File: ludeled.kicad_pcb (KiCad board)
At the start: 2 copper layers, 379 parts, among them U1 ESP32-WROOM-32E

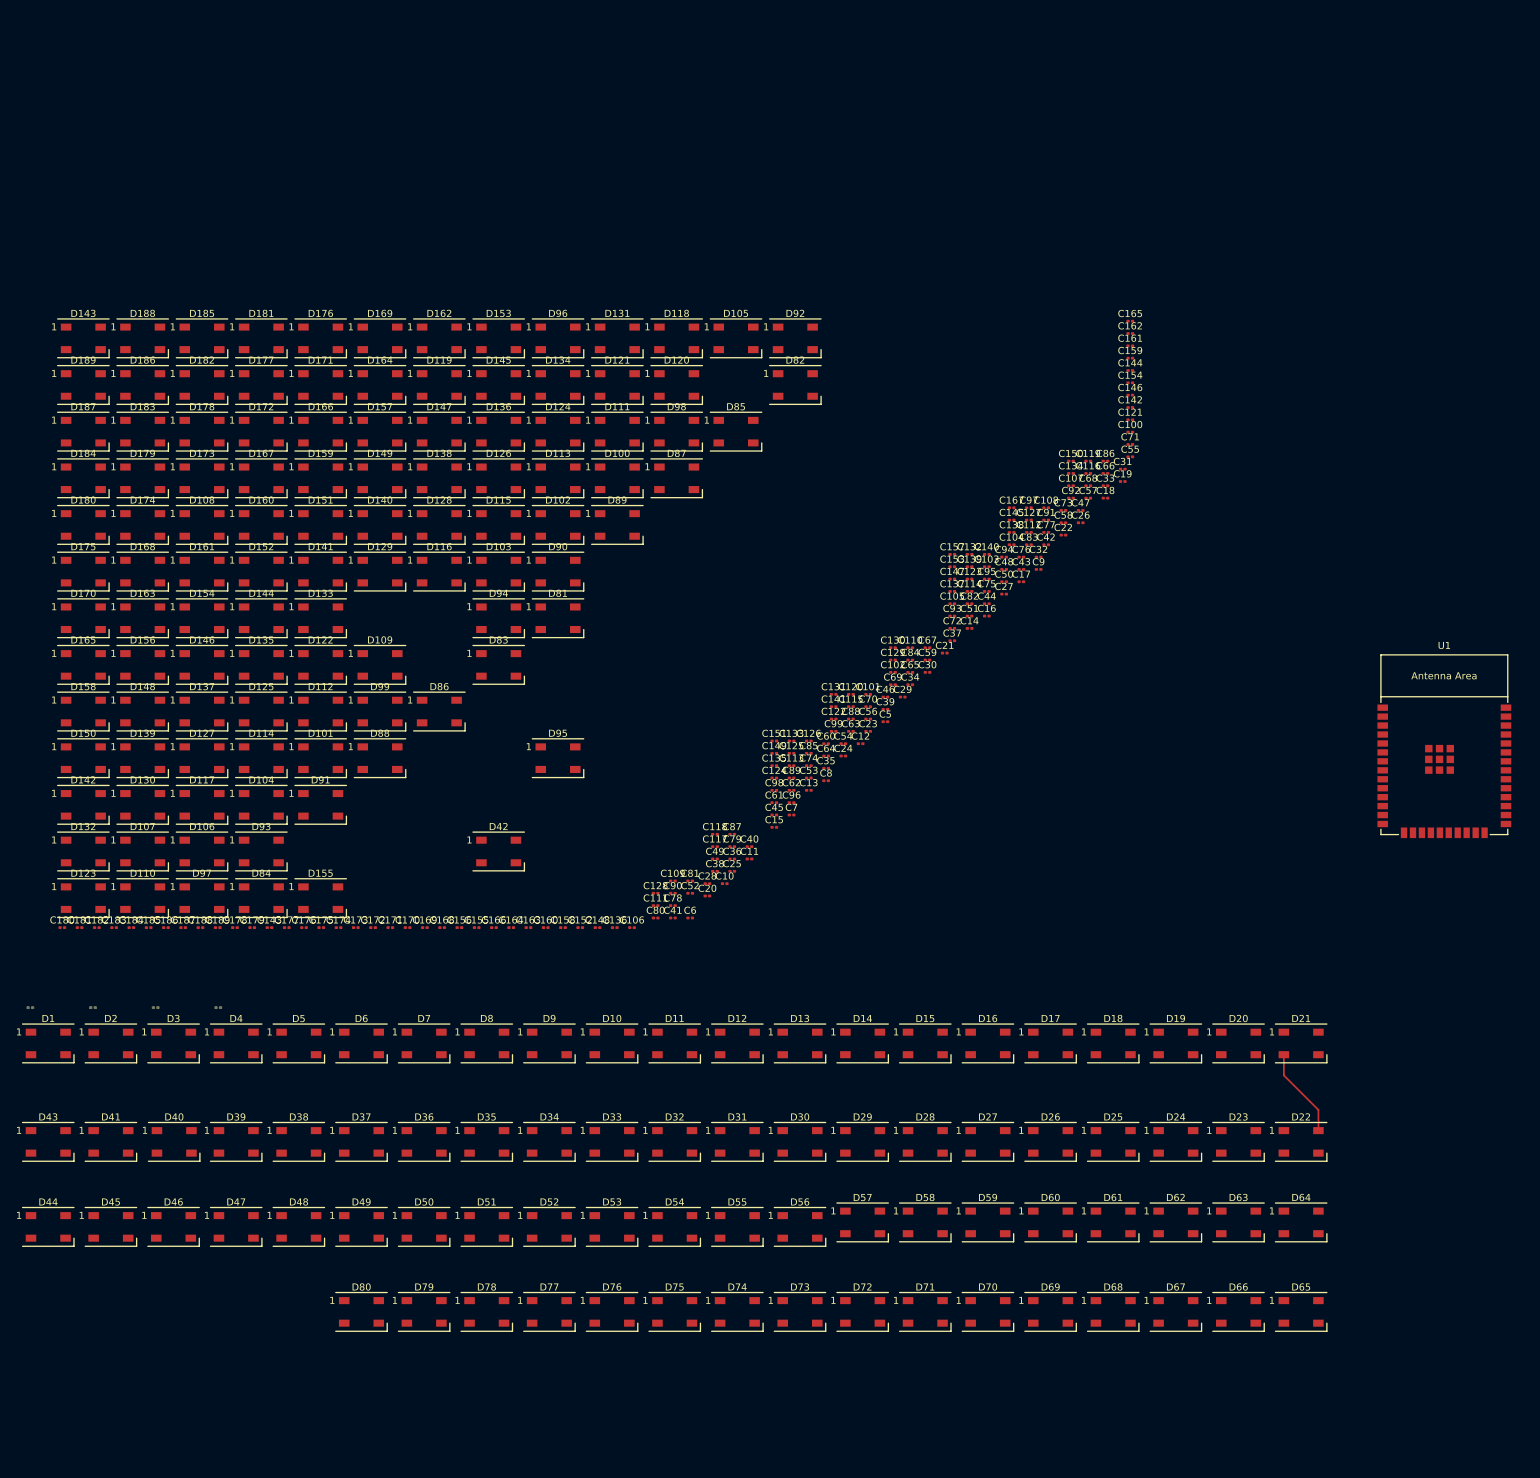
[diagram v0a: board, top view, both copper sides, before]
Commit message: More layout
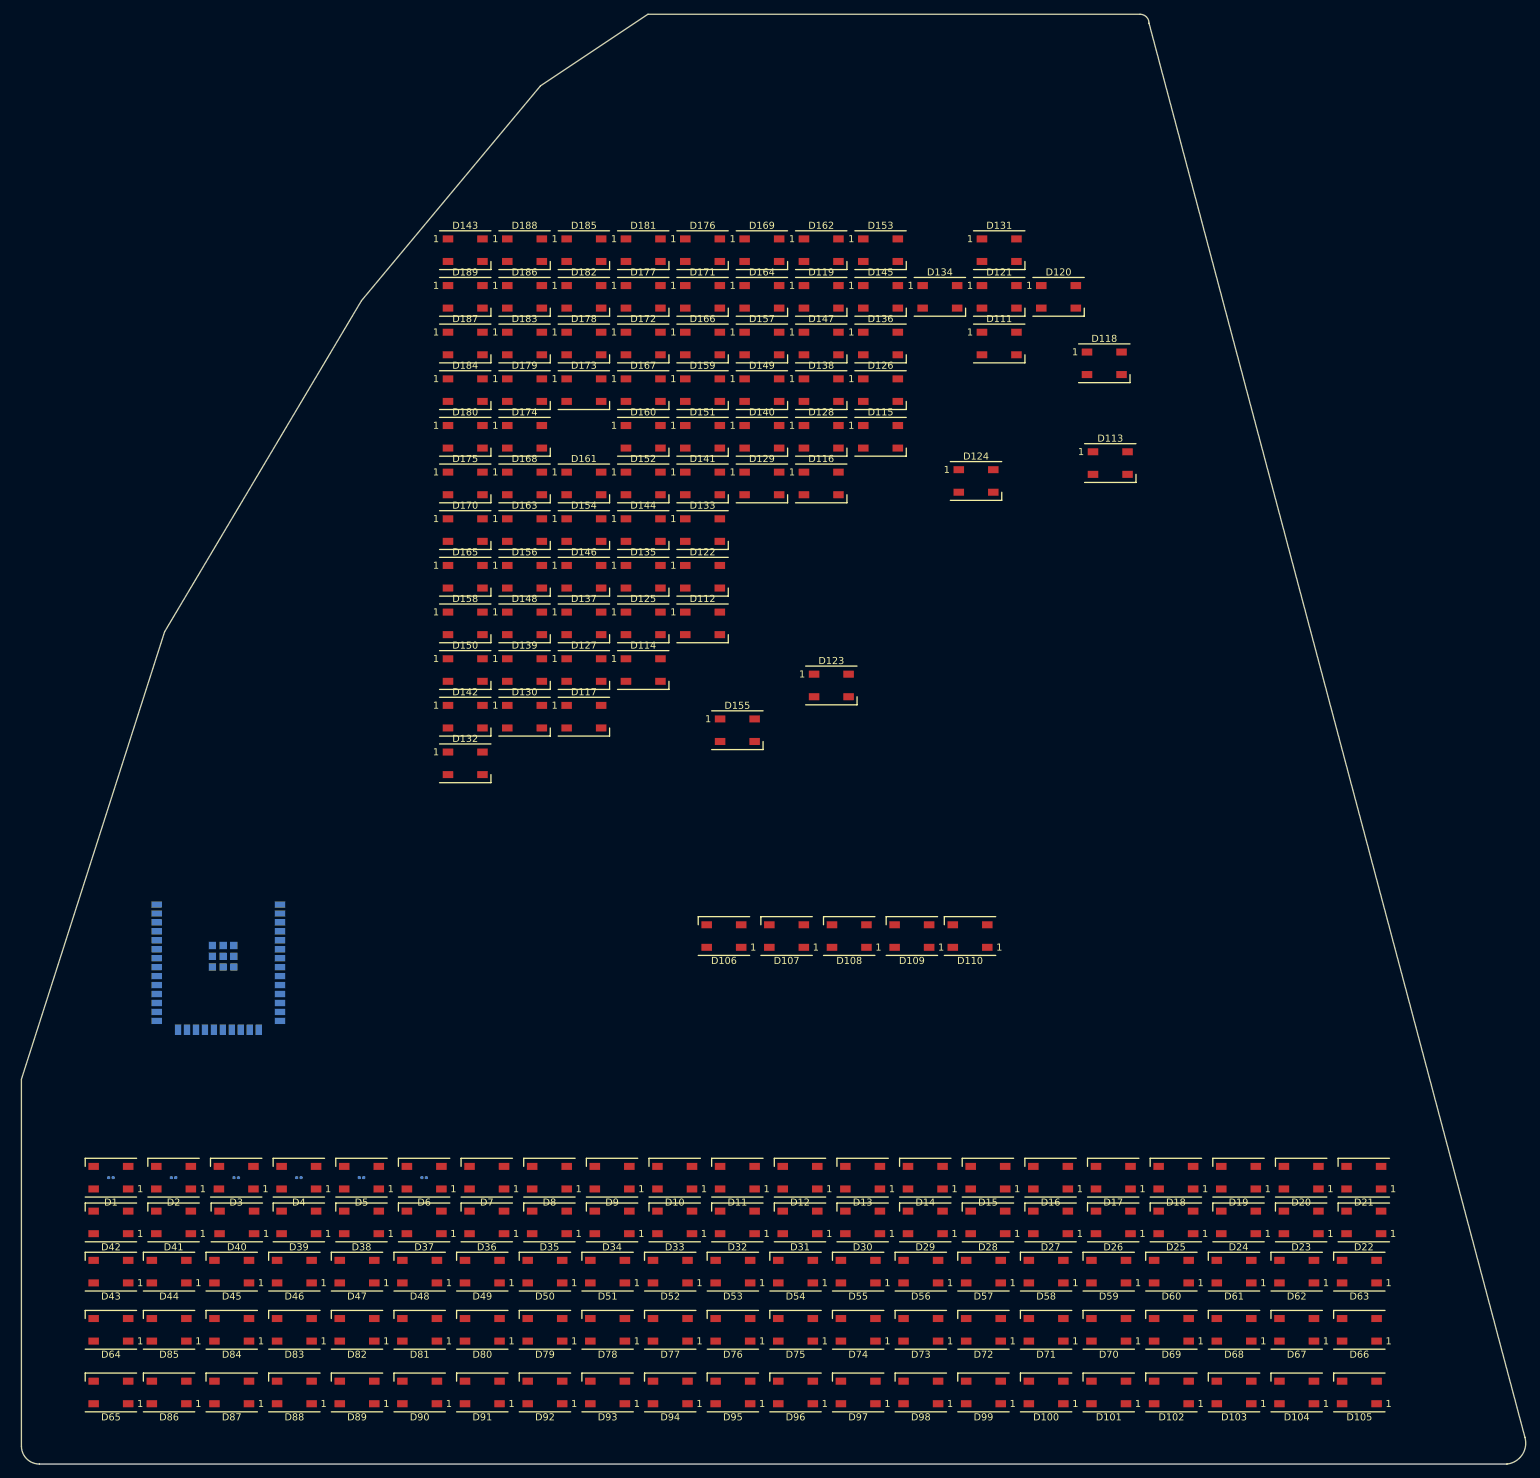
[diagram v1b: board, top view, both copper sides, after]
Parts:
- removed C10, C100, C101, C102, C103, C104, C105, C106, C107, C108, C109, C11, C110, C111, C112, C113, C114, C115, C116, C117, C118, C119, C12, C120, C121, C122, C123, C124, C125, C126, C127, C128, C129, C13, C130, C131, C132, C133, C134, C135, C136, C137, C138, C139, C14, C140, C141, C142, C143, C144, C145, C146, C147, C148, C149, C15, C150, C151, C152, C153, C154, C155, C156, C157, C158, C159, C16, C160, C161, C162, C163, C164, C165, C166, C167, C168, C169, C17, C170, C171, C172, C173, C174, C175, C176, C177, C178, C179, C18, C180, C181, C182, C183, C184, C185, C186, C187, C188, C189, C19, C20, C21, C22, C23, C24, C25, C26, C27, C28, C29, C30, C31, C32, C33, C34, C35, C36, C37, C38, C39, C40, C41, C42, C43, C44, C45, C46, C47, C48, C49, C50, C51, C52, C53, C54, C55, C56, C57, C58, C59, C60, C61, C62, C63, C64, C65, C66, C67, C68, C69, C7, C70, C71, C72, C73, C74, C75, C76, C77, C78, C79, C8, C80, C81, C82, C83, C84, C85, C86, C87, C88, C89, C9, C90, C91, C92, C93, C94, C95, C96, C97, C98, C99: 100nF, Capacitor_SMD:C_0201_0603Metric
- C5, C6, U1: moved to B.Cu
- moved U1 176.2 mm to (64.8, 74.9), turned to 180 degrees
- moved D105 173.8 mm to (226.7, 137.2), turned to 180 degrees
- moved D64 169.6 mm to (49.5, 128.3), turned to 180 degrees
- moved D65 169.3 mm to (49.5, 137.2), turned to 180 degrees
- moved D104 168.9 mm to (217.8, 137.2), turned to 180 degrees
- moved D103 156.4 mm to (208.9, 137.2), turned to 180 degrees
- moved D92 153.8 mm to (111.1, 137.2), turned to 180 degrees
- moved D96 153.3 mm to (146.7, 137.2), turned to 180 degrees
- moved D102 150.8 mm to (200.0, 137.2), turned to 180 degrees
- moved D85 150.7 mm to (57.8, 128.3), turned to 180 degrees
- moved D82 147.8 mm to (84.5, 128.3), turned to 180 degrees
- moved D87 144.3 mm to (66.7, 137.2), turned to 180 degrees
- moved D101 143.6 mm to (191.1, 137.2), turned to 180 degrees
- moved D100 143.3 mm to (182.2, 137.2), turned to 180 degrees
- moved D98 140.7 mm to (164.5, 137.2), turned to 180 degrees
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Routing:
- net Net-(D21-Pad2): track 12.8 -> 0.00 mm
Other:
- board outline added: 213.5 x 205.7 mm

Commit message: layout done
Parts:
- added C7: 100nF, Capacitor_SMD:C_0201_0603Metric, F.Cu at (134.1, 16.8)
- added C8: 100nF, Capacitor_SMD:C_0201_0603Metric, F.Cu at (142.3, 16.8)
- added C9: 100nF, Capacitor_SMD:C_0201_0603Metric, F.Cu at (150.7, 16.8)
- added D190: WS2812B, LED_SMD:LED_WS2812B_PLCC4_5.0x5.0mm_P3.2mm, F.Cu at (98.5, 113.0)
- added D191: WS2812B, LED_SMD:LED_WS2812B_PLCC4_5.0x5.0mm_P3.2mm, F.Cu at (106.8, 113.0)
- added D192: WS2812B, LED_SMD:LED_WS2812B_PLCC4_5.0x5.0mm_P3.2mm, F.Cu at (115.0, 113.0)
- added D193: WS2812B, LED_SMD:LED_WS2812B_PLCC4_5.0x5.0mm_P3.2mm, F.Cu at (123.2, 113.0)
- added D194: WS2812B, LED_SMD:LED_WS2812B_PLCC4_5.0x5.0mm_P3.2mm, F.Cu at (131.5, 113.0)
- added D195: WS2812B, LED_SMD:LED_WS2812B_PLCC4_5.0x5.0mm_P3.2mm, F.Cu at (139.8, 113.0)
- added D196: WS2812B, LED_SMD:LED_WS2812B_PLCC4_5.0x5.0mm_P3.2mm, F.Cu at (148.0, 113.0)
- added D197: WS2812B, LED_SMD:LED_WS2812B_PLCC4_5.0x5.0mm_P3.2mm, F.Cu at (156.2, 113.0)
- added D198: WS2812B, LED_SMD:LED_WS2812B_PLCC4_5.0x5.0mm_P3.2mm, F.Cu at (164.5, 113.0)
- added D199: WS2812B, LED_SMD:LED_WS2812B_PLCC4_5.0x5.0mm_P3.2mm, F.Cu at (172.8, 113.0)
- added D200: WS2812B, LED_SMD:LED_WS2812B_PLCC4_5.0x5.0mm_P3.2mm, F.Cu at (7.50, 121.2)
- added D201: WS2812B, LED_SMD:LED_WS2812B_PLCC4_5.0x5.0mm_P3.2mm, F.Cu at (15.8, 121.2)
- added D202: WS2812B, LED_SMD:LED_WS2812B_PLCC4_5.0x5.0mm_P3.2mm, F.Cu at (24.0, 121.2)
- added D203: WS2812B, LED_SMD:LED_WS2812B_PLCC4_5.0x5.0mm_P3.2mm, F.Cu at (32.2, 121.2)
- added D204: WS2812B, LED_SMD:LED_WS2812B_PLCC4_5.0x5.0mm_P3.2mm, F.Cu at (40.5, 121.2)
- added D205: WS2812B, LED_SMD:LED_WS2812B_PLCC4_5.0x5.0mm_P3.2mm, F.Cu at (48.8, 121.2)
- added D206: WS2812B, LED_SMD:LED_WS2812B_PLCC4_5.0x5.0mm_P3.2mm, F.Cu at (57.0, 121.2)
- added D207: WS2812B, LED_SMD:LED_WS2812B_PLCC4_5.0x5.0mm_P3.2mm, F.Cu at (65.2, 121.2)
- added D208: WS2812B, LED_SMD:LED_WS2812B_PLCC4_5.0x5.0mm_P3.2mm, F.Cu at (73.5, 121.2)
- added D209: WS2812B, LED_SMD:LED_WS2812B_PLCC4_5.0x5.0mm_P3.2mm, F.Cu at (81.8, 121.2)
- added D210: WS2812B, LED_SMD:LED_WS2812B_PLCC4_5.0x5.0mm_P3.2mm, F.Cu at (90.0, 121.2)
- added D211: WS2812B, LED_SMD:LED_WS2812B_PLCC4_5.0x5.0mm_P3.2mm, F.Cu at (98.2, 121.2)
- added D212: WS2812B, LED_SMD:LED_WS2812B_PLCC4_5.0x5.0mm_P3.2mm, F.Cu at (106.5, 121.2)
- added D213: WS2812B, LED_SMD:LED_WS2812B_PLCC4_5.0x5.0mm_P3.2mm, F.Cu at (115.0, 121.2)
- added D214: WS2812B, LED_SMD:LED_WS2812B_PLCC4_5.0x5.0mm_P3.2mm, F.Cu at (123.2, 121.2)
- added D215: WS2812B, LED_SMD:LED_WS2812B_PLCC4_5.0x5.0mm_P3.2mm, F.Cu at (131.8, 121.2)
- added D216: WS2812B, LED_SMD:LED_WS2812B_PLCC4_5.0x5.0mm_P3.2mm, F.Cu at (140.0, 121.2)
- added D217: WS2812B, LED_SMD:LED_WS2812B_PLCC4_5.0x5.0mm_P3.2mm, F.Cu at (148.2, 121.2)
- added D218: WS2812B, LED_SMD:LED_WS2812B_PLCC4_5.0x5.0mm_P3.2mm, F.Cu at (156.5, 121.2)
- added D219: WS2812B, LED_SMD:LED_WS2812B_PLCC4_5.0x5.0mm_P3.2mm, F.Cu at (164.8, 121.2)
- added D220: WS2812B, LED_SMD:LED_WS2812B_PLCC4_5.0x5.0mm_P3.2mm, F.Cu at (173.0, 121.2)
- added D221: WS2812B, LED_SMD:LED_WS2812B_PLCC4_5.0x5.0mm_P3.2mm, F.Cu at (7.50, 129.5)
- added D222: WS2812B, LED_SMD:LED_WS2812B_PLCC4_5.0x5.0mm_P3.2mm, F.Cu at (15.8, 129.5)
- added D223: WS2812B, LED_SMD:LED_WS2812B_PLCC4_5.0x5.0mm_P3.2mm, F.Cu at (24.1, 129.5)
- added D224: WS2812B, LED_SMD:LED_WS2812B_PLCC4_5.0x5.0mm_P3.2mm, F.Cu at (32.4, 129.5)
- added D225: WS2812B, LED_SMD:LED_WS2812B_PLCC4_5.0x5.0mm_P3.2mm, F.Cu at (40.7, 129.5)
- added D226: WS2812B, LED_SMD:LED_WS2812B_PLCC4_5.0x5.0mm_P3.2mm, F.Cu at (49.0, 129.5)
- added D227: WS2812B, LED_SMD:LED_WS2812B_PLCC4_5.0x5.0mm_P3.2mm, F.Cu at (57.3, 129.5)
- added D228: WS2812B, LED_SMD:LED_WS2812B_PLCC4_5.0x5.0mm_P3.2mm, F.Cu at (65.6, 129.5)
- added D229: WS2812B, LED_SMD:LED_WS2812B_PLCC4_5.0x5.0mm_P3.2mm, F.Cu at (73.9, 129.5)
- added D230: WS2812B, LED_SMD:LED_WS2812B_PLCC4_5.0x5.0mm_P3.2mm, F.Cu at (82.2, 129.5)
- added D231: WS2812B, LED_SMD:LED_WS2812B_PLCC4_5.0x5.0mm_P3.2mm, F.Cu at (90.5, 129.5)
- added D232: WS2812B, LED_SMD:LED_WS2812B_PLCC4_5.0x5.0mm_P3.2mm, F.Cu at (98.8, 129.5)
- added D233: WS2812B, LED_SMD:LED_WS2812B_PLCC4_5.0x5.0mm_P3.2mm, F.Cu at (107.1, 129.5)
- added D234: WS2812B, LED_SMD:LED_WS2812B_PLCC4_5.0x5.0mm_P3.2mm, F.Cu at (115.4, 129.5)
- added D235: WS2812B, LED_SMD:LED_WS2812B_PLCC4_5.0x5.0mm_P3.2mm, F.Cu at (123.7, 129.5)
- added D236: WS2812B, LED_SMD:LED_WS2812B_PLCC4_5.0x5.0mm_P3.2mm, F.Cu at (132.0, 129.5)
- added D237: WS2812B, LED_SMD:LED_WS2812B_PLCC4_5.0x5.0mm_P3.2mm, F.Cu at (140.3, 129.5)
- added D238: WS2812B, LED_SMD:LED_WS2812B_PLCC4_5.0x5.0mm_P3.2mm, F.Cu at (148.6, 129.5)
- added D239: WS2812B, LED_SMD:LED_WS2812B_PLCC4_5.0x5.0mm_P3.2mm, F.Cu at (156.9, 129.5)
- added D240: WS2812B, LED_SMD:LED_WS2812B_PLCC4_5.0x5.0mm_P3.2mm, F.Cu at (165.2, 129.5)
- added D241: WS2812B, LED_SMD:LED_WS2812B_PLCC4_5.0x5.0mm_P3.2mm, F.Cu at (173.5, 129.5)
- added D242: WS2812B, LED_SMD:LED_WS2812B_PLCC4_5.0x5.0mm_P3.2mm, F.Cu at (7.50, 137.8)
- added D243: WS2812B, LED_SMD:LED_WS2812B_PLCC4_5.0x5.0mm_P3.2mm, F.Cu at (15.8, 137.8)
- added D244: WS2812B, LED_SMD:LED_WS2812B_PLCC4_5.0x5.0mm_P3.2mm, F.Cu at (24.1, 137.8)
- added D245: WS2812B, LED_SMD:LED_WS2812B_PLCC4_5.0x5.0mm_P3.2mm, F.Cu at (32.4, 137.8)
- added D246: WS2812B, LED_SMD:LED_WS2812B_PLCC4_5.0x5.0mm_P3.2mm, F.Cu at (40.7, 137.8)
- added D247: WS2812B, LED_SMD:LED_WS2812B_PLCC4_5.0x5.0mm_P3.2mm, F.Cu at (49.0, 137.8)
- added D248: WS2812B, LED_SMD:LED_WS2812B_PLCC4_5.0x5.0mm_P3.2mm, F.Cu at (57.3, 137.8)
- added D249: WS2812B, LED_SMD:LED_WS2812B_PLCC4_5.0x5.0mm_P3.2mm, F.Cu at (65.6, 137.8)
- added D250: WS2812B, LED_SMD:LED_WS2812B_PLCC4_5.0x5.0mm_P3.2mm, F.Cu at (73.9, 137.8)
- added D251: WS2812B, LED_SMD:LED_WS2812B_PLCC4_5.0x5.0mm_P3.2mm, F.Cu at (82.2, 137.8)
- added D252: WS2812B, LED_SMD:LED_WS2812B_PLCC4_5.0x5.0mm_P3.2mm, F.Cu at (90.5, 137.8)
- added D253: WS2812B, LED_SMD:LED_WS2812B_PLCC4_5.0x5.0mm_P3.2mm, F.Cu at (98.8, 137.8)
- added D254: WS2812B, LED_SMD:LED_WS2812B_PLCC4_5.0x5.0mm_P3.2mm, F.Cu at (107.1, 137.8)
- added D255: WS2812B, LED_SMD:LED_WS2812B_PLCC4_5.0x5.0mm_P3.2mm, F.Cu at (115.4, 137.8)
- added D256: WS2812B, LED_SMD:LED_WS2812B_PLCC4_5.0x5.0mm_P3.2mm, F.Cu at (123.7, 137.8)
- added D257: WS2812B, LED_SMD:LED_WS2812B_PLCC4_5.0x5.0mm_P3.2mm, F.Cu at (132.0, 137.8)
- added D258: WS2812B, LED_SMD:LED_WS2812B_PLCC4_5.0x5.0mm_P3.2mm, F.Cu at (140.3, 137.8)
- added D259: WS2812B, LED_SMD:LED_WS2812B_PLCC4_5.0x5.0mm_P3.2mm, F.Cu at (148.6, 137.8)
- added D260: WS2812B, LED_SMD:LED_WS2812B_PLCC4_5.0x5.0mm_P3.2mm, F.Cu at (156.9, 137.8)
- added D261: WS2812B, LED_SMD:LED_WS2812B_PLCC4_5.0x5.0mm_P3.2mm, F.Cu at (165.2, 137.8)
- added D262: WS2812B, LED_SMD:LED_WS2812B_PLCC4_5.0x5.0mm_P3.2mm, F.Cu at (173.5, 137.8)
- added D263: WS2812B, LED_SMD:LED_WS2812B_PLCC4_5.0x5.0mm_P3.2mm, F.Cu at (181.8, 137.8)
- C1, C2, C3, C4, C5, C6: moved to F.Cu
- moved D105 210.5 mm to (24.1, 79.8)
- moved D162 175.4 mm to (32.2, 104.8), turned to 180 degrees
- moved D21 171.4 mm to (74.0, 30.0)
- moved D181 171.0 mm to (24.0, 113.0), turned to 180 degrees
- moved D20 170.9 mm to (65.8, 30.0)
- moved D22 167.2 mm to (82.2, 30.0)
- moved D124 161.4 mm to (32.2, 88.0), turned to 180 degrees
- moved D145 159.0 mm to (48.8, 96.5), turned to 180 degrees
- moved D182 156.1 mm to (32.2, 113.0), turned to 180 degrees
- moved D72 155.2 mm to (32.5, 63.2)
- moved D164 154.2 mm to (49.0, 104.8), turned to 180 degrees
- moved D23 152.5 mm to (90.5, 30.0)
- moved D63 151.0 mm to (90.5, 54.9)
- moved D62 150.4 mm to (82.2, 54.9)
- moved D160 150.3 mm to (15.8, 104.8), turned to 180 degrees
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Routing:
- net Net-(D30-Pad2): track 0.00 -> 100.6 mm
- net Net-(D19-Pad2): track 0.00 -> 92.7 mm
- net Net-(D10-Pad4): track 0.00 -> 84.1 mm
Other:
- board size 213.5 x 205.7 mm -> 190 x 140 mm
